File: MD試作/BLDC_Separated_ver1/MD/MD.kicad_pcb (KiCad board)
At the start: 4 copper layers, 35 x 35 mm, 68 parts, among them J4 Conn_02x13_Odd_Even, J5 Conn_01x02_Pin, J6 Conn_01x03_Pin, Q10 TPN19008QM, Q11 TPN19008QM, Q12 TPN19008QM, Q2 DI035P04PT, Q5 BSS138, Q6 DI035P04PT, Q7 TPN19008QM, Q8 TPN19008QM, Q9 TPN19008QM, SW4 SW_SPDT, U6 Driver_FETGate_DRV8323S

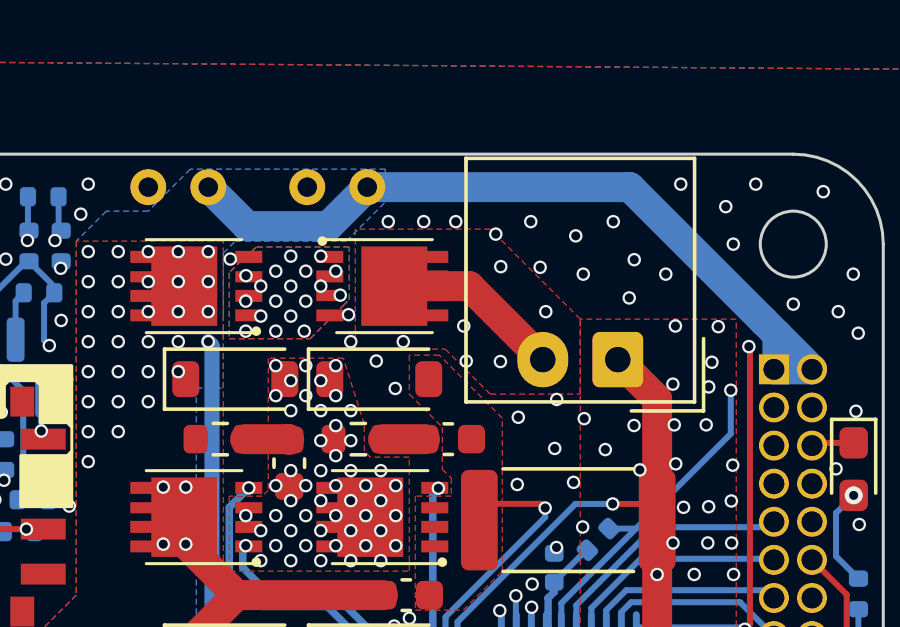
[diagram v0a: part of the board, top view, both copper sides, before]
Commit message: 発注後修正1
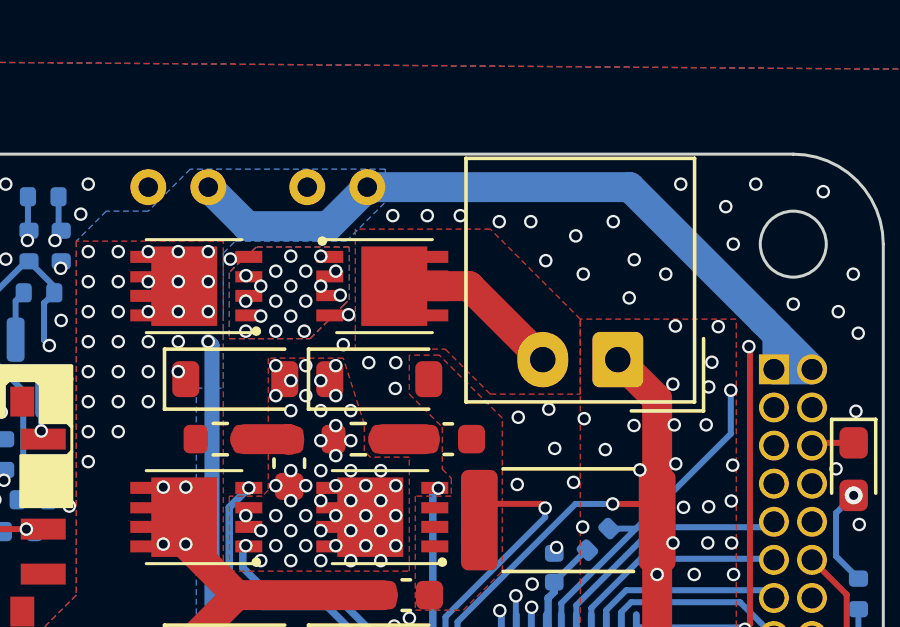
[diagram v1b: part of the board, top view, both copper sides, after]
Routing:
- net GND: vias 217 -> 212
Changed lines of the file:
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@@
   (via (at 29.303917 28.013254) (size 0.45) (drill 0.3) (layers "F.Cu" "B.Cu") (free) (net 4))
   (via (at 22.75 34) (size 0.45) (drill 0.3) (layers "F.Cu" "B.Cu") (free) (net 4))
-  (via (at 18.100705 6.895796) (size 0.45) (drill 0.3) (layers "F.Cu" "B.Cu") (free) (net 4))
+  (via (at 17.85 6.95) (size 0.45) (drill 0.3) (layers "F.Cu" "B.Cu") (free) (net 4))
   (via (at 25.468466 18.011122) (size 0.45) (drill 0.3) (layers "F.Cu" "B.Cu") (net 4))
   (via (at 7.866903 11.731696) (size 0.45) (drill 0.3) (layers "F.Cu" "B.Cu") (free) (net 4))
@@
   (via (at 26.698716 3.51793) (size 0.45) (drill 0.3) (layers "F.Cu" "B.Cu") (free) (net 4))
   (via (at 29.982009 10.367076) (size 0.45) (drill 0.3) (layers "F.Cu" "B.Cu") (free) (net 4))
-  (via (at 23.75 5.25) (size 0.45) (drill 0.3) (layers "F.Cu" "B.Cu") (free) (net 4))
   (via (at 28.27476 24.821045) (size 0.45) (drill 0.3) (layers "F.Cu" "B.Cu") (free) (net 4))
   (via (at 18.733451 7.810217) (size 0.45) (drill 0.3) (layers "F.Cu" "B.Cu") (free) (net 4))
@@
   (via (at 1.8 33.6) (size 0.45) (drill 0.3) (layers "F.Cu" "B.Cu") (free) (net 4))
   (via (at 8.25 2) (size 0.45) (drill 0.3) (layers "F.Cu" "B.Cu") (free) (net 4))
-  (via (at 21.015422 5.729515) (size 0.45) (drill 0.3) (layers "F.Cu" "B.Cu") (free) (net 4))
   (via (at 26.959631 29.371422) (size 0.45) (drill 0.3) (layers "F.Cu" "B.Cu") (net 4))
   (via (at 33.25 33.5) (size 0.45) (drill 0.3) (layers "F.Cu" "B.Cu") (free) (net 4))
@@
   (via (at 29.173765 21.402366) (size 0.45) (drill 0.3) (layers "F.Cu" "B.Cu") (free) (net 4))
   (via (at 28.266181 21.415332) (size 0.45) (drill 0.3) (layers "F.Cu" "B.Cu") (free) (net 4))
-  (via (at 22.238945 6.912995) (size 0.45) (drill 0.3) (layers "F.Cu" "B.Cu") (free) (net 4))
   (via (at 28.082808 10.323724) (size 0.45) (drill 0.3) (layers "F.Cu" "B.Cu") (net 4))
   (via (at 29.946357 12.960821) (size 0.45) (drill 0.3) (layers "F.Cu" "B.Cu") (free) (net 4))
-  (via (at 20.75 2.25) (size 0.45) (drill 0.3) (layers "F.Cu" "B.Cu") (free) (net 4))
+  (via (at 20.9 2.05) (size 0.45) (drill 0.3) (layers "F.Cu" "B.Cu") (free) (net 4))
   (via (at 24.962349 28.116426) (size 0.45) (drill 0.3) (layers "F.Cu" "B.Cu") (free) (net 4))
   (via (at 7.595912 5.543687) (size 0.45) (drill 0.3) (layers "F.Cu" "B.Cu") (free) (net 4))
@@
   (via (at 28.668345 27.424521) (size 0.45) (drill 0.3) (layers "F.Cu" "B.Cu") (free) (net 4))
   (via (at 30 34) (size 0.45) (drill 0.3) (layers "F.Cu" "B.Cu") (free) (net 4))
-  (via (at 21.099956 6.899647) (size 0.45) (drill 0.3) (layers "F.Cu" "B.Cu") (free) (net 4))
   (via (at 22.990265 18.090221) (size 0.45) (drill 0.3) (layers "F.Cu" "B.Cu") (net 4))
   (via (at 19.204805 15.468521) (size 0.45) (drill 0.3) (layers "F.Cu" "B.Cu") (free) (net 4))
@@
   (via (at 2 8.8) (size 0.45) (drill 0.3) (layers "F.Cu" "B.Cu") (free) (net 4))
   (via (at 32 29.2) (size 0.45) (drill 0.3) (layers "F.Cu" "B.Cu") (free) (net 4))
-  (via (at 17.25 6.25) (size 0.45) (drill 0.3) (layers "F.Cu" "B.Cu") (free) (net 4))
+  (via (at 17 6.35) (size 0.45) (drill 0.3) (layers "F.Cu" "B.Cu") (free) (net 4))
   (via (at 22.972721 32.233427) (size 0.45) (drill 0.3) (layers "F.Cu" "B.Cu") (free) (net 4))
   (via (at 29.398304 24.244577) (size 0.45) (drill 0.3) (layers "F.Cu" "B.Cu") (free) (net 4))
@@
   (via (at 29.935007 11.561298) (size 0.45) (drill 0.3) (layers "F.Cu" "B.Cu") (free) (net 4))
   (via (at 27.005545 31.70541) (size 0.45) (drill 0.3) (layers "F.Cu" "B.Cu") (net 4))
-  (via (at 24.114795 8.176756) (size 0.45) (drill 0.3) (layers "F.Cu" "B.Cu") (free) (net 4))
+  (via (at 23.85 8.5) (size 0.45) (drill 0.3) (layers "F.Cu" "B.Cu") (free) (net 4))
   (via (at 26.618399 20.085403) (size 0.45) (drill 0.3) (layers "F.Cu" "B.Cu") (free) (net 4))
-  (via (at 19.681317 2.249359) (size 0.45) (drill 0.3) (layers "F.Cu" "B.Cu") (free) (net 4))
-  (via (at 18.5 2.25) (size 0.45) (drill 0.3) (layers "F.Cu" "B.Cu") (free) (net 4))
+  (via (at 19.8 2.05) (size 0.45) (drill 0.3) (layers "F.Cu" "B.Cu") (free) (net 4))
+  (via (at 18.65 2.05) (size 0.45) (drill 0.3) (layers "F.Cu" "B.Cu") (free) (net 4))
   (via (at 10.8 33.4) (size 0.45) (drill 0.3) (layers "F.Cu" "B.Cu") (free) (net 4))
   (via (at 28.033289 9.024165) (size 0.45) (drill 0.3) (layers "F.Cu" "B.Cu") (net 4))
@@
   (via (at 25.491054 29.998255) (size 0.45) (drill 0.3) (layers "F.Cu" "B.Cu") (free) (net 4))
   (via (at 26.885587 10.524244) (size 0.45) (drill 0.3) (layers "F.Cu" "B.Cu") (net 4))
-  (via (at 23.562945 3.772711) (size 0.45) (drill 0.3) (layers "F.Cu" "B.Cu") (free) (net 4))
+  (via (at 23.75 3.55) (size 0.45) (drill 0.3) (layers "F.Cu" "B.Cu") (free) (net 4))
   (via (at 28.269516 22.210886) (size 0.45) (drill 0.3) (layers "F.Cu" "B.Cu") (free) (net 4))
   (via (at 2 4.75) (size 0.45) (drill 0.3) (layers "F.Cu" "B.Cu") (free) (net 4))
@@
   (via (at 27.510605 32.256384) (size 0.45) (drill 0.3) (layers "F.Cu" "B.Cu") (net 4))
   (via (at 27.75 4) (size 0.45) (drill 0.3) (layers "F.Cu" "B.Cu") (free) (net 4))
-  (via (at 22.083254 2.665392) (size 0.45) (drill 0.3) (layers "F.Cu" "B.Cu") (free) (net 4))
+  (via (at 22.2 2.25) (size 0.45) (drill 0.3) (layers "F.Cu" "B.Cu") (free) (net 4))
   (via (at 29.75 1.75) (size 0.45) (drill 0.3) (layers "F.Cu" "B.Cu") (free) (net 4))
   (via (at 30.75 1) (size 0.45) (drill 0.3) (layers "F.Cu" "B.Cu") (free) (net 4))
@@
   (via (at 24.462839 28.770109) (size 0.45) (drill 0.3) (layers "F.Cu" "B.Cu") (net 4))
   (via (at 28.070936 5.728687) (size 0.45) (drill 0.3) (layers "F.Cu" "B.Cu") (free) (net 4))
-  (via (at 19 6.25) (size 0.45) (drill 0.3) (layers "F.Cu" "B.Cu") (free) (net 4))
+  (via (at 18.75 6.95) (size 0.45) (drill 0.3) (layers "F.Cu" "B.Cu") (free) (net 4))
   (via (at 23.048628 20.491082) (size 0.45) (drill 0.3) (layers "F.Cu" "B.Cu") (net 4))
   (via (at 28.28779 23.148385) (size 0.45) (drill 0.3) (layers "F.Cu" "B.Cu") (free) (net 4))
@@
   (via (at 24.380766 32.317603) (size 0.45) (drill 0.3) (layers "F.Cu" "B.Cu") (free) (net 4))
   (via (at 29.5 5.75) (size 0.45) (drill 0.3) (layers "F.Cu" "B.Cu") (free) (net 4))
-  (via (at 22.25 3.75) (size 0.45) (drill 0.3) (layers "F.Cu" "B.Cu") (free) (net 4))
   (via (at 26.612896 17.004243) (size 0.45) (drill 0.3) (layers "F.Cu" "B.Cu") (free) (net 4))
   (via (at 28.75808 23.568373) (size 0.45) (drill 0.3) (layers "F.Cu" "B.Cu") (free) (net 4))
@@
   )
   (zone (net 25) (net_name "/Power/24VBAT") (layer "F.Cu") (hatch edge 0.5)
+    (priority 1)
     (connect_pads yes (clearance 0.2))
     (min_thickness 0.25) (filled_areas_thickness no)
